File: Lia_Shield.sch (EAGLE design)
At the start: 9 parts, among them U1 HC_05

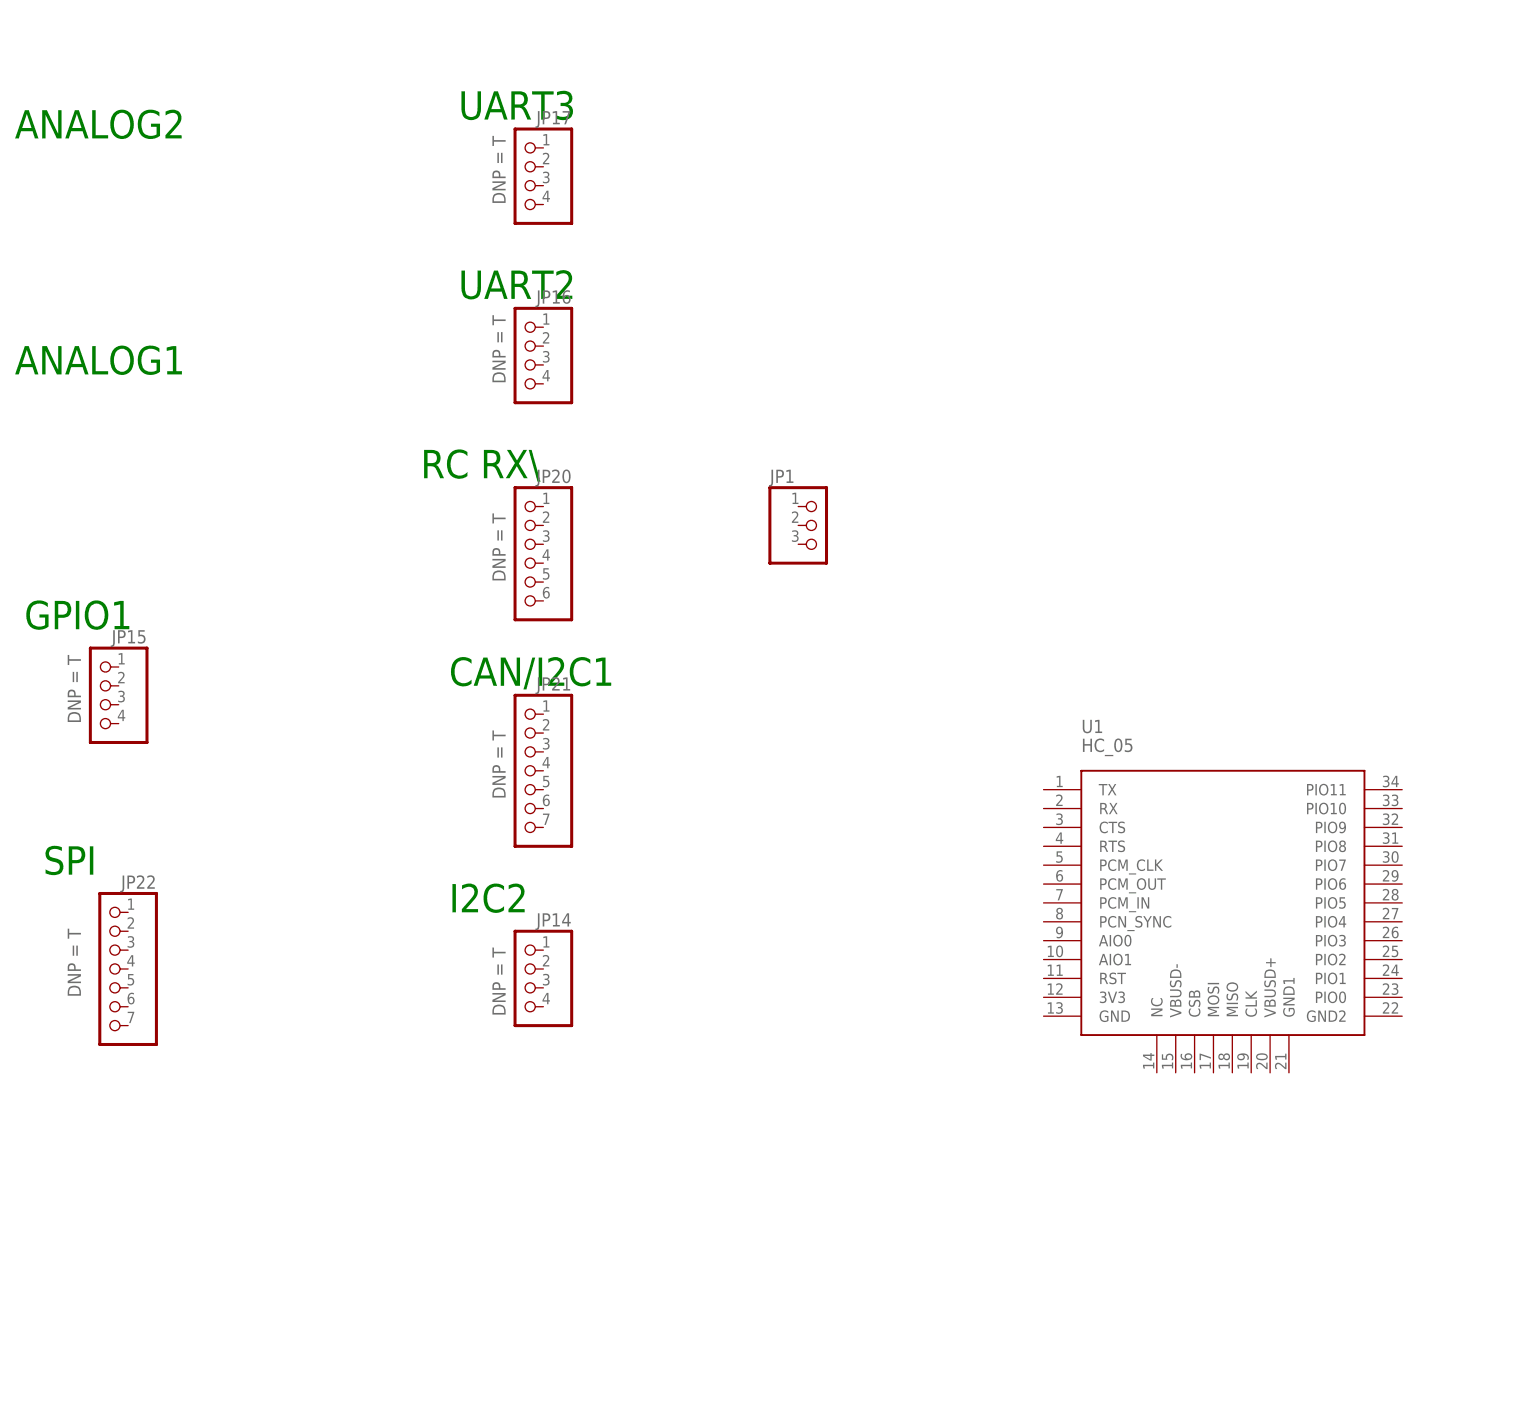
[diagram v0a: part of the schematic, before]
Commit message: david wollte es so
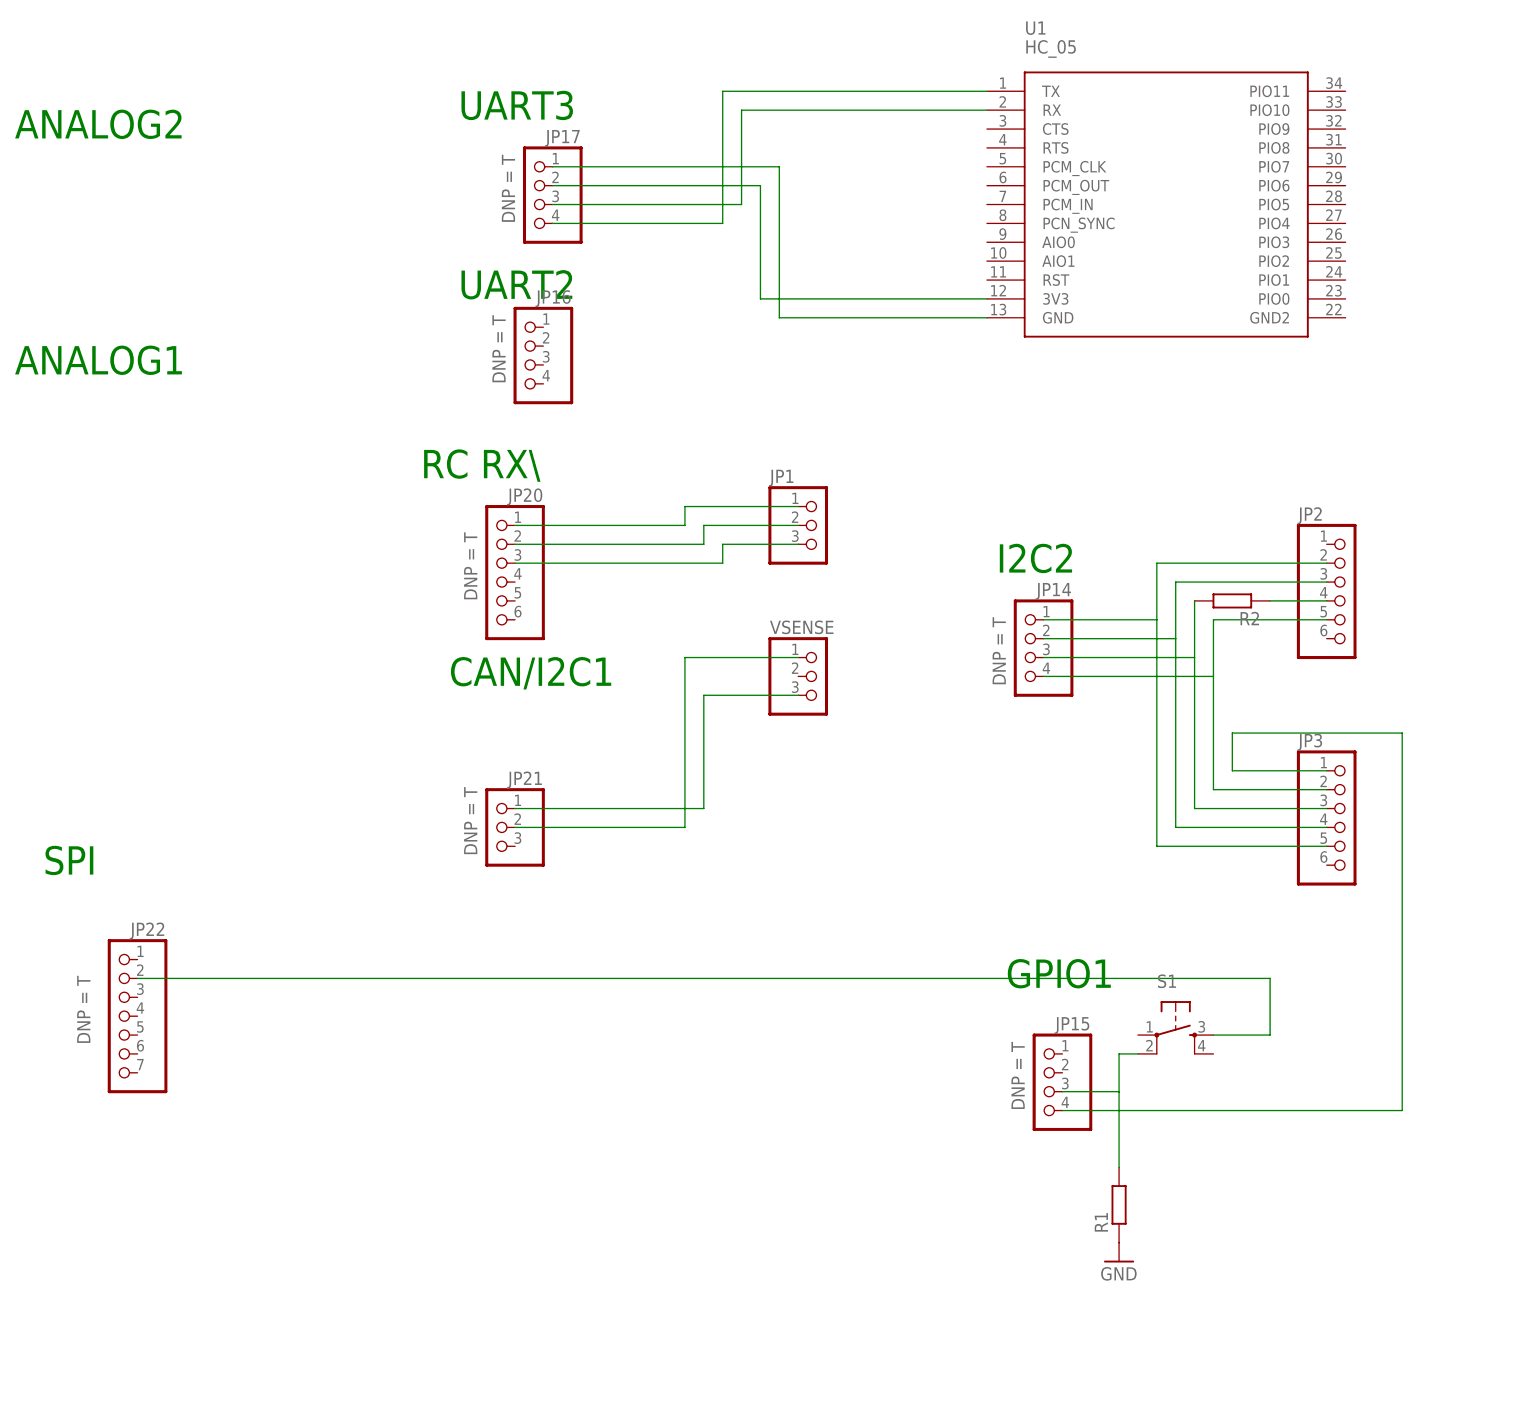
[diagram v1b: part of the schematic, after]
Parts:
- added JP2, JP3: (no value), pinhead:PINHD-1X6
- added R1, R2: (no value), rcl:R-EU_R1206
- added S1: (no value), SparkFun-Electromechanical:TAC_SWITCHPTH
- added VSENSE: (no value), pinhead:PINHD-1X3/90
- JP21: device pinhead:PINHD-1X7 -> pinhead:PINHD-1X3
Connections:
- new net GND: R1.1
- new net N$1: JP21.2, VSENSE.1
- new net N$10: JP14.3, JP3.3, R2.2
- new net N$11: JP14.1, JP2.2, JP3.5
- new net N$12: JP14.2, JP2.3, JP3.4
- new net N$13: JP14.4, JP2.5, JP3.2
- new net N$14: JP15.4, JP3.1
- new net N$15: JP22.2, S1.3
- new net N$16: JP15.3, R1.2, S1.2
- new net N$17: JP2.4, R2.1
- new net N$2: JP1.1, JP20.1
- new net N$3: JP21.1, VSENSE.3
- new net N$4: JP17.1, U1.GND
- new net N$5: JP1.2, JP20.2
- new net N$6: JP1.3, JP20.3
- new net N$7: JP17.2, U1.3V3
- new net N$8: JP17.3, U1.RX
- new net N$9: JP17.4, U1.TX
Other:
- moved on the sheet: JP14, JP15, JP17, JP20, JP22
